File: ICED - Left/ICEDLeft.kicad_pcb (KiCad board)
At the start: 2 copper layers, 175.4 x 145.5 mm, 162 parts, among them P1 FLASH_HDR, P2 USB3_MICRO, P3 CONN_17, P4 USB3_AFEMALE, Q1 TC1264, U1 MK20DX256VLH7, U2 IS31FL3731C, X1 CRYSTAL

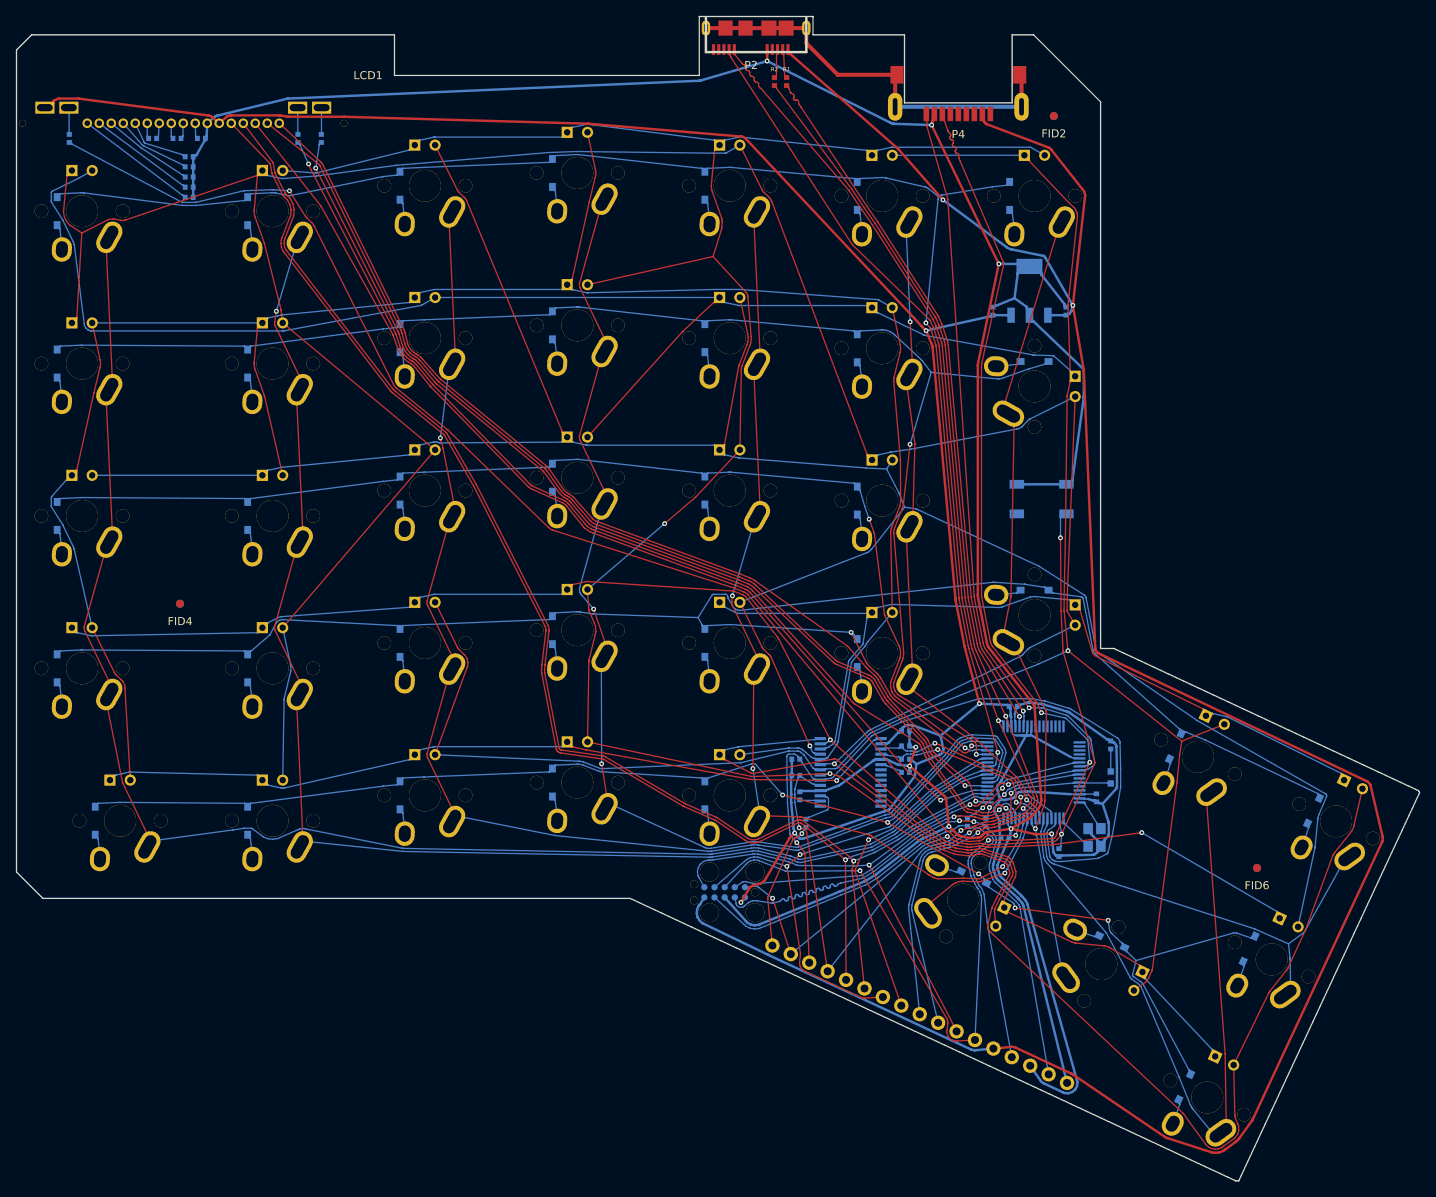
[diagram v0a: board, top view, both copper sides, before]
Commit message: ICED 1.2b, now with 100% more Type C
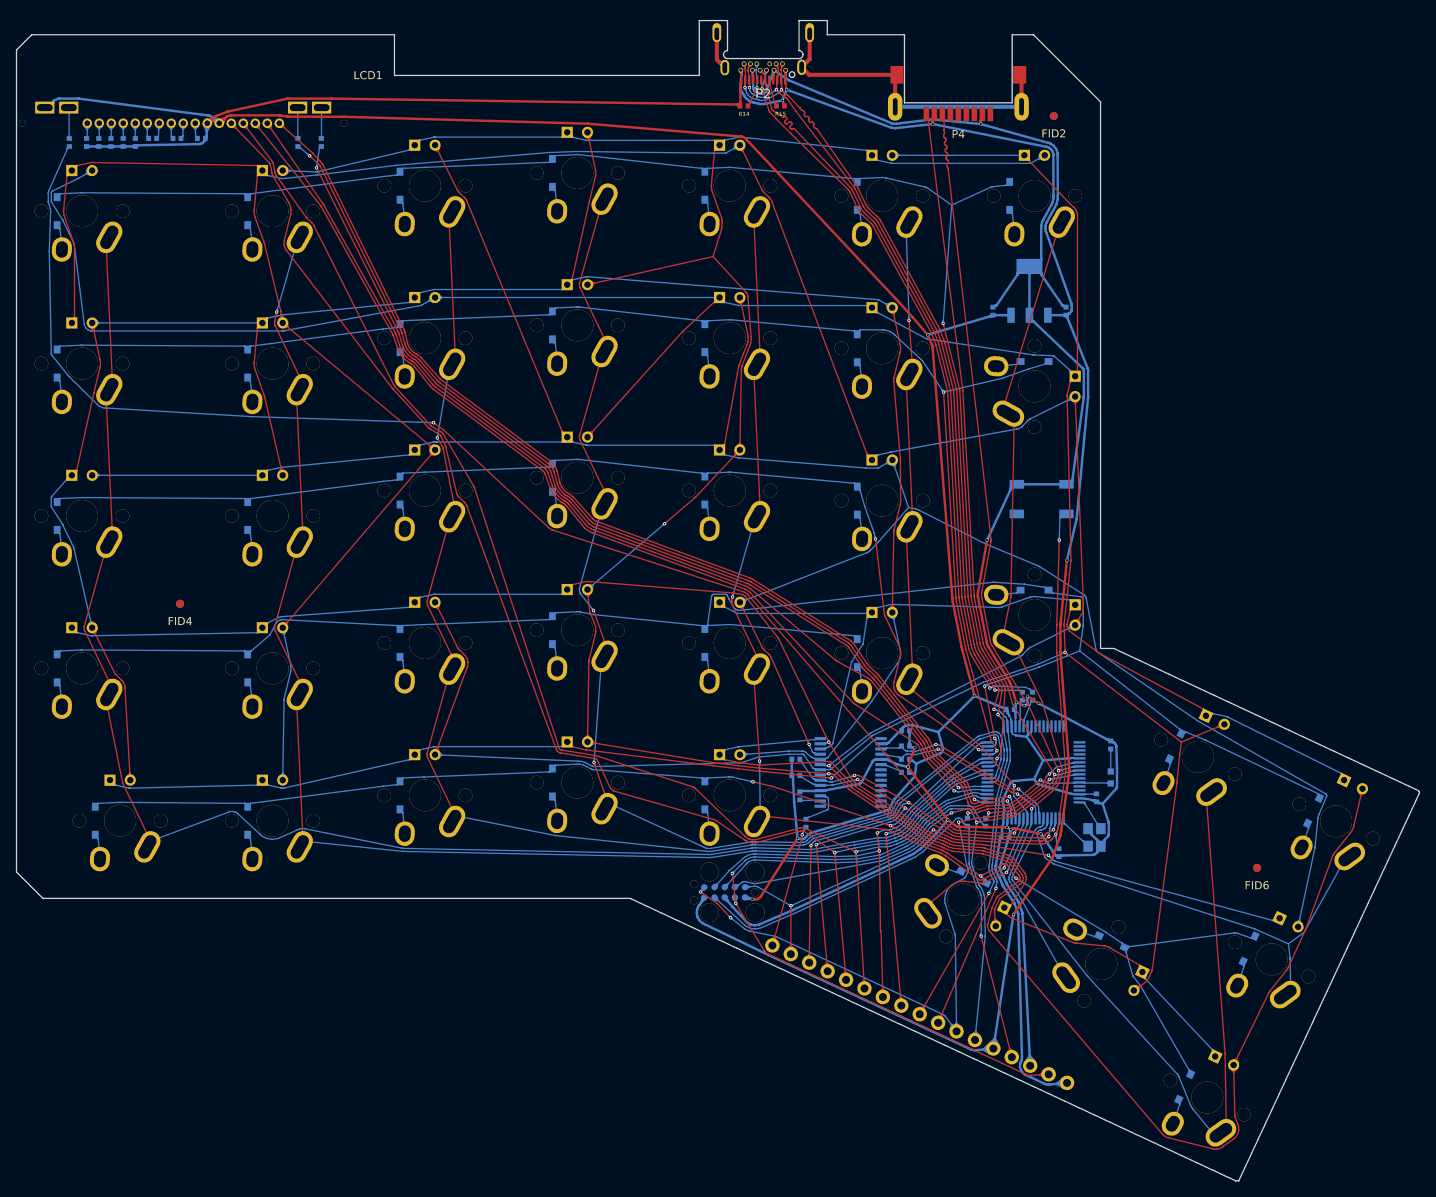
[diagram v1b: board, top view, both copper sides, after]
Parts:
- added R14: 5.1k, prettylib:SMD-1005, F.Cu at (108.6, 36.4)
- added R15: 5.1k, prettylib:SMD-1005, F.Cu at (113.2, 36.4)
- P2: value USB3_MICRO -> USBC; footprint prettylib:USB3_MICROB_STAKES -> prettylib:USB_C_MIDMOUNT_TH_IMPCUT
- R1, R2: moved to B.Cu
- moved R2 83.3 mm to (144.7, 110.2), turned to 180 degrees
- moved R1 82.3 mm to (143.4, 110.2), turned to 180 degrees
- moved C17 14.5 mm to (26.4, 41.0), turned to 0 degrees
- moved C16 12.6 mm to (27.9, 41.0), turned to 0 degrees
- moved C15 10.7 mm to (29.5, 41.0), turned to 0 degrees
- moved C14 8.80 mm to (31.0, 41.0), turned to 0 degrees
- moved P2 7.43 mm to (111.0, 32.5)
- moved C13 6.96 mm to (32.5, 41.0), turned to 0 degrees
- moved C4 0.54 mm to (141.9, 111.9)
- moved R10 0.51 mm to (52.8, 41.0)
- moved R13 0.51 mm to (24.3, 41.0)
- moved R9 0.51 mm to (55.8, 41.0)
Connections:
- net /mcu/PTB18 renamed /Col3
- net /mcu/PTB19 renamed /Col4
- net /mcu/PTB2 renamed /Col1
- net /mcu/PTB3 renamed /Col2
- net /mcu/PTC0 renamed /Col5
- net /mcu/PTC10 renamed /Col7
- net /mcu/PTC11 renamed /Col8
- net /mcu/PTC9 renamed /Col6
- net /mcu/PTD0 renamed /Col9
- net /mcu/PTD1 renamed /Row1
- net /mcu/PTD4 renamed /Row2
- net /mcu/PTD5 renamed /Row3
- net /mcu/PTD6 renamed /Row4
- net /mcu/PTD7 renamed /Row5
- P2 pad 1: +5V -> VSS
- P2 pad 10: (no net) -> /mcu/RX1
- P2 pad 11: /mcu/GND -> /mcu/TX1
- P2 pad 2: Net-(P2-Pad2) -> /mcu/TX1
- P2 pad 3: Net-(P2-Pad3) -> /mcu/RX1
- P2 pad 4: (no net) -> +5V
- P2 pad 5: VSS -> Net-(P2-Pad5)
- P2 pad 6: /mcu/RX1 -> /mcu/USB_DP
- P2 pad 7: /mcu/TX1 -> /mcu/USB_DM
- P2 pad 8: (no net) -> Net-(P2-Pad8)
- P2 pad 9: (no net) -> +5V
- P4 pad 10: /mcu/GND -> /GND
- P4 pad 2: (no net) -> Net-(P4-Pad2)
- P4 pad 3: (no net) -> Net-(P4-Pad3)
- P4 pad 7: (no net) -> Net-(P4-Pad7)
- P4 pad 8: (no net) -> Net-(P4-Pad8)
- P4 pad 9: (no net) -> Net-(P4-Pad9)
- R1 pad 1: Net-(P2-Pad2) -> /mcu/USB_DP
- R1 pad 2: /mcu/USB_DM -> Net-(R1-Pad2)
- R2 pad 1: Net-(P2-Pad3) -> /mcu/USB_DM
- R2 pad 2: /mcu/USB_DP -> Net-(R2-Pad2)
- S39 pad 1: (no net) -> Net-(S39-Pad1)
- U1 pad 10: (no net) -> /mcu/ADC0_DM0
- U1 pad 11: (no net) -> /mcu/ADC1_DP0
- U1 pad 12: (no net) -> /mcu/ADC1_DM0
- U1 pad 13: (no net) -> Net-(U1-Pad13)
- U1 pad 14: (no net) -> Net-(U1-Pad14)
- U1 pad 15: (no net) -> Net-(U1-Pad15)
- U1 pad 16: (no net) -> Net-(U1-Pad16)
- U1 pad 17: (no net) -> Net-(U1-Pad17)
- U1 pad 18: (no net) -> Net-(U1-Pad18)
- U1 pad 19: (no net) -> Net-(U1-Pad19)
- U1 pad 20: (no net) -> Net-(U1-Pad20)
- U1 pad 26: (no net) -> /mcu/PTA4
- U1 pad 28: (no net) -> /mcu/PTA12
- U1 pad 29: (no net) -> /mcu/PTA13
- U1 pad 5: /mcu/USB_DP -> Net-(R1-Pad2)
- U1 pad 6: /mcu/USB_DM -> Net-(R2-Pad2)
- U1 pad 9: (no net) -> /mcu/ADC0_DP0
- U2 pad 10: (no net) -> /mcu/CB4
- U2 pad 11: (no net) -> /mcu/CB5
- U2 pad 12: (no net) -> /mcu/CB6
- U2 pad 13: (no net) -> /mcu/CB7
- U2 pad 14: (no net) -> /mcu/CB8
- U2 pad 15: (no net) -> /mcu/CB9
- U2 pad 7: (no net) -> /mcu/CB1
- U2 pad 8: (no net) -> /mcu/CB2
- U2 pad 9: (no net) -> /mcu/CB3
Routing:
- net +5V: track 292.8 -> 218.9 mm, vias 2 -> 3
- net /mcu/GND: track 51.4 -> 0.00 mm
- net /GND: track 0.00 -> 45.5 mm
- net /mcu/SCL0: track 101.5 -> 72.1 mm, vias 1 -> 4
- net /ledmatrix/CA3: track 368.4 -> 389.0 mm
- net /ledmatrix/CA1: track 357.0 -> 376.8 mm
- net VSS: track 419.3 -> 399.5 mm, vias 8 -> 14
- net /mcu/SWD_DIO: track 72.4 -> 91.7 mm
- net /ledmatrix/CA4: track 273.0 -> 288.6 mm
- net /mcu/LCD_KR: track 159.9 -> 174.0 mm
- net /ledmatrix/CA2: track 418.0 -> 431.6 mm
- net Net-(C17-Pad2): track 15.4 -> 3.08 mm
- net /ledmatrix/CA5: track 297.7 -> 309.3 mm
- net /mcu/RX0: track 182.1 -> 171.1 mm, vias 4 -> 2
- net Net-(C16-Pad2): track 13.4 -> 3.08 mm
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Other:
- board size 175.4 x 145.5 mm -> 175.4 x 145 mm
- net class 4mil added: clearance 0.1016, trace_width 0.1016, via_dia 0.4064, via_drill 0.2032
- net class Default: clearance 0.1524 -> 0.1016; via_dia 0.6096 -> 0.4064; via_drill 0.3048 -> 0.2032
- net class GND: clearance 0.1524 -> 0.1016
- net class Power: clearance 0.1524 -> 0.1016
- rule pad_to_mask_clearance: 0.0762 -> 0.0508
- rule trace_clearance: 0.1524 -> 0.1016
- rule via_min_drill: 0.3048 -> 0.2032
- rule via_min_size: 0.508 -> 0.4064
- board text added: "ICED-L Rev 1.2b Batch __"
- board text removed: "ICED-L Rev 1.1d Batch __"
